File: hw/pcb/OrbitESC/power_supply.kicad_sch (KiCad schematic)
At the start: 31 parts, among them J11 VDC, J12 GND, Q7 2N7002, U7 AP62200Z6-7, U8 AP2171W, U9 AP2120

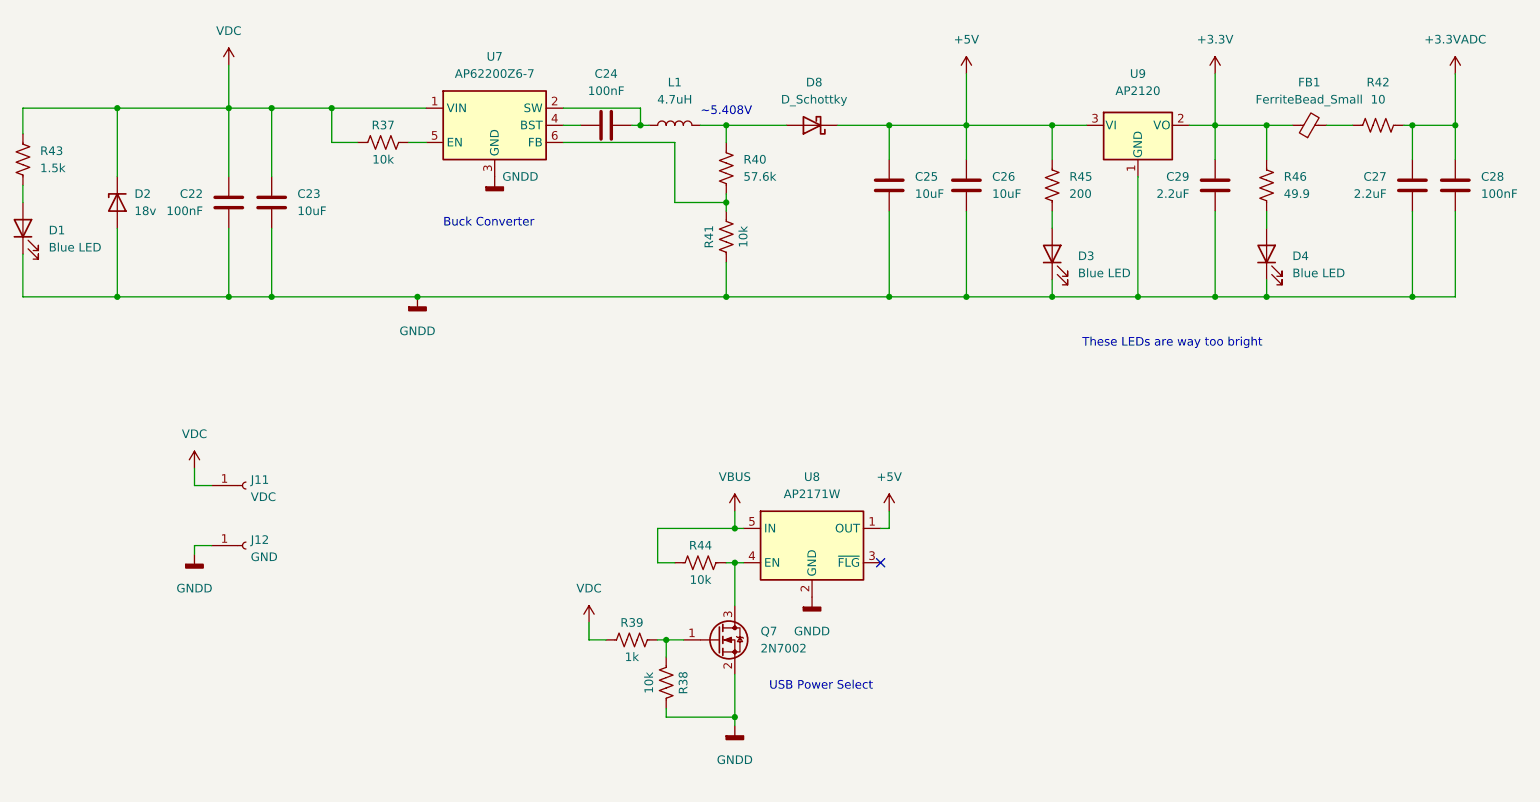
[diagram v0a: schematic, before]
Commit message: Sync lunch schematic update
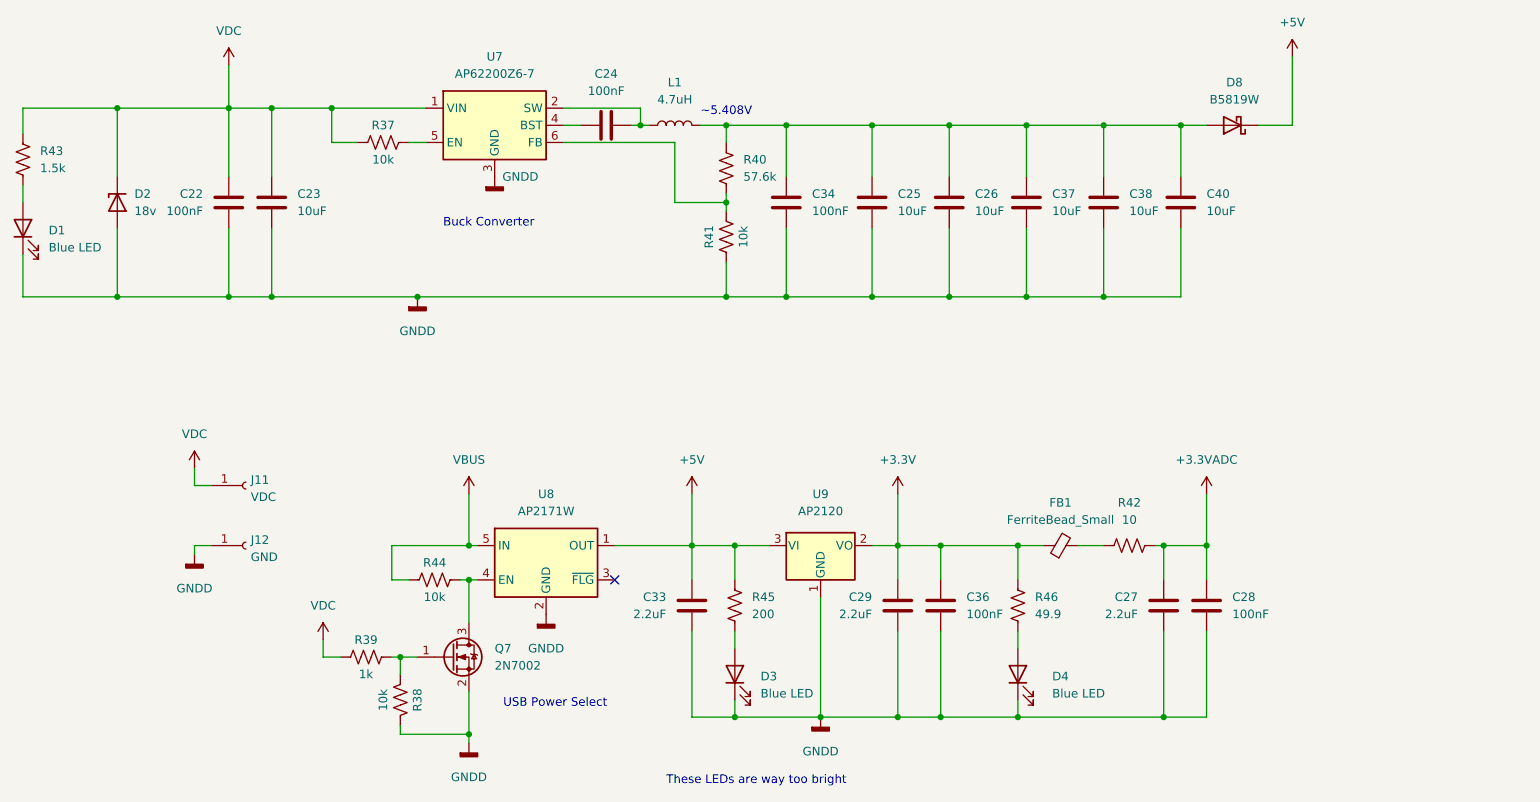
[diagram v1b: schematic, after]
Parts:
- added C33: 2.2uF, Capacitor_SMD:C_0805_2012Metric, symbol Device:C
- added C34, C36: 100nF, Capacitor_SMD:C_0402_1005Metric, symbol Device:C
- added C37, C38, C40: 10uF, Capacitor_SMD:C_0805_2012Metric, symbol Device:C
- D8: value D_Schottky -> B5819W; footprint (none) -> Diode_SMD:D_SOD-123; JLCPCB (none) -> C8598
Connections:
- net +3.3V: now also C36.1
- net +5V: now also C33.2; no longer C25.1, C26.1
- net GNDD: now also C33.1, C34.2, C36.2, C37.2, C38.2, C40.2
- net at D8.2 (A), L1.2, R40.1: now also C25.1, C26.1, C34.1, C37.1, C38.1, C40.1
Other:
- moved on the sheet: C25, C26, C27, C28, C29, D3, D4, D8, FB1, Q7, R38, R39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
